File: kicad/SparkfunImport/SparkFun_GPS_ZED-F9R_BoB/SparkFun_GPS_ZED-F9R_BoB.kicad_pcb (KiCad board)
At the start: 2 copper layers, 43.2 x 50.8 mm, 145 parts, among them J1 U.FL, J2 USB_C_2-LAYER_PADS, J3 QWIIC_RIGHT_ANGLE, J4 QWIIC_RIGHT_ANGLE, J5 CONN_111X11_NO_SILK, J6 CONN_09NO_SILK, J7 CONN_06NO_SILK_NO_POP, U1 DUAL-OPTO_HCPL-073L, U2 U-BLOX_ZED_F9R, U3 UHS_INVERTER_SCHMITT_TRIGGERS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, U4 UHS_INVERTER_SCHMITT_TRIGGERS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, U5 V_REG_AP2112K-3.3V

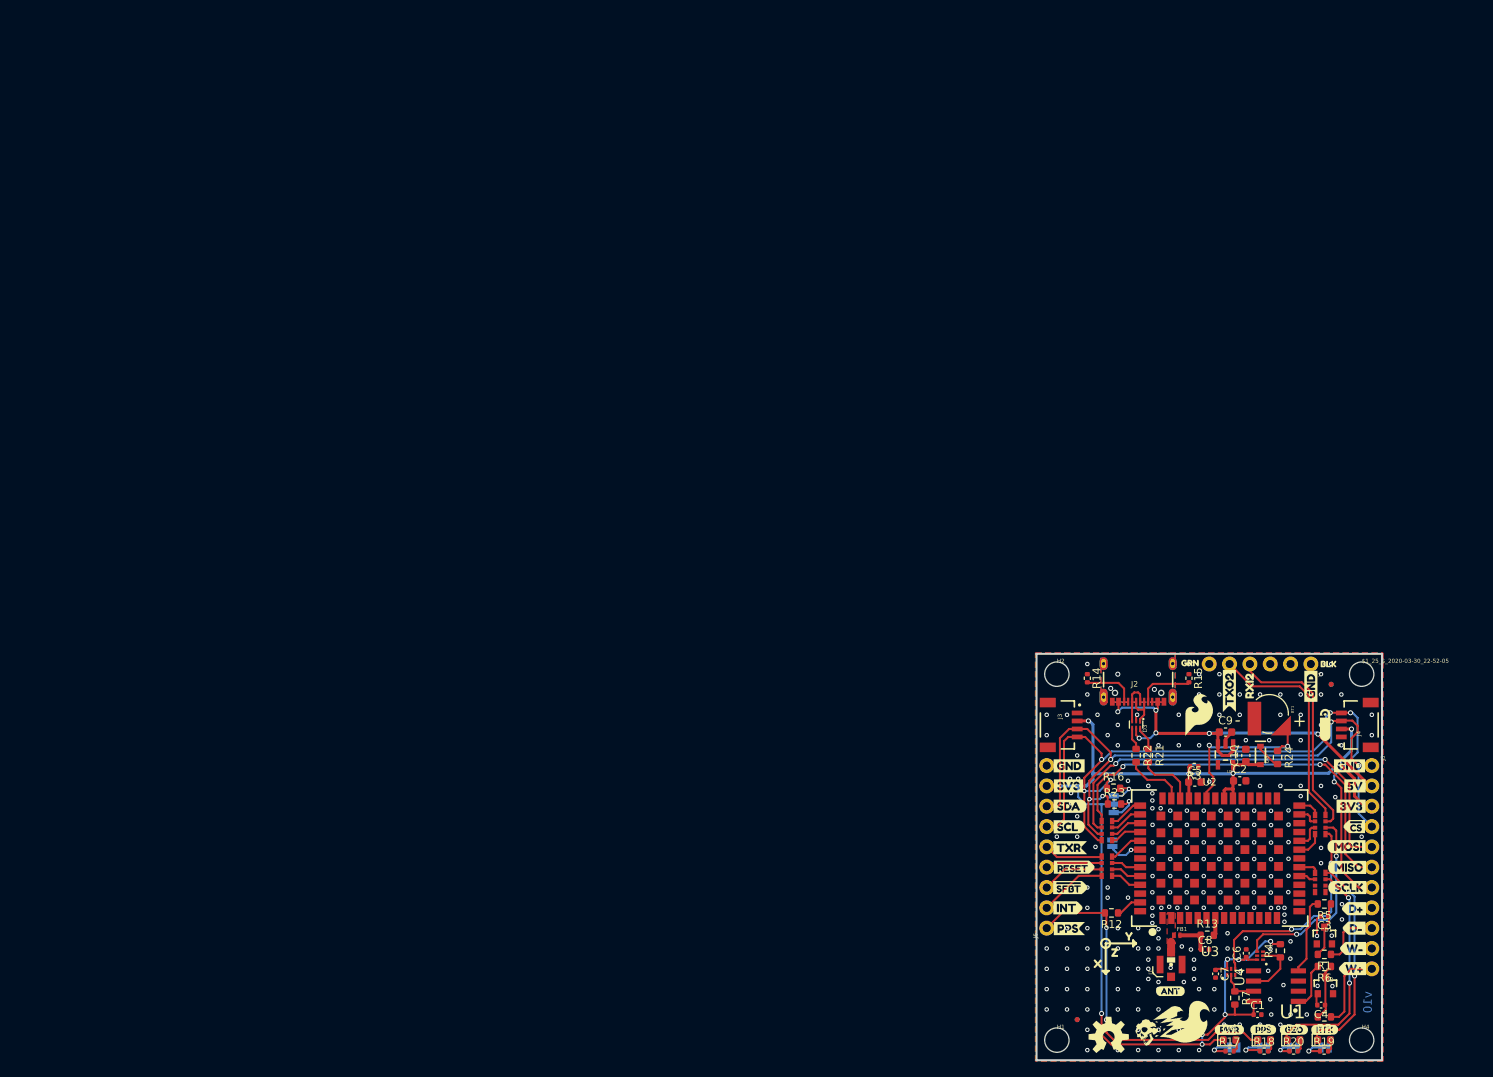
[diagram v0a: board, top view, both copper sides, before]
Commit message: Starting to make gps_breakout
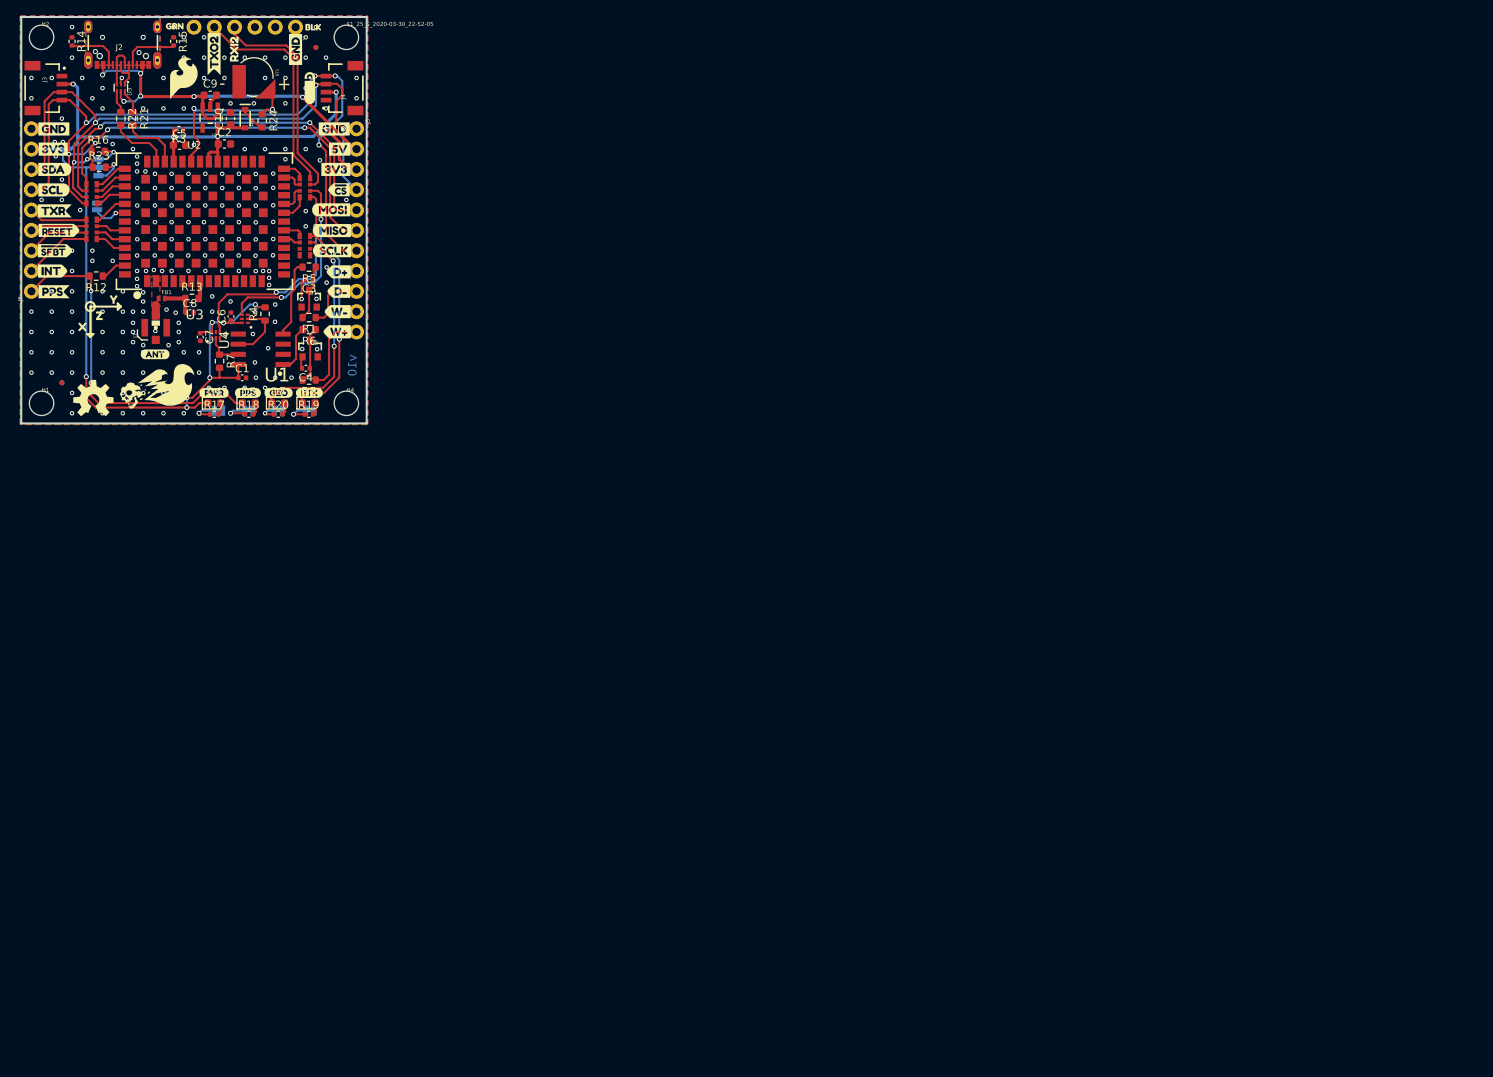
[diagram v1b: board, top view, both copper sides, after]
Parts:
- moved BT1 149.8 mm to (29.1, 7.49)
- moved C1 149.8 mm to (27.6, 45.1)
- moved C10 149.8 mm to (26.2, 12.7)
- moved C2 149.8 mm to (25.4, 15.9)
- moved C3 149.8 mm to (36.0, 32.8)
- moved C4 149.8 mm to (35.6, 43.9)
- moved C5 149.8 mm to (19.8, 16.0)
- moved C6 149.8 mm to (26.2, 37.4)
- moved C8 149.8 mm to (21.1, 37.0)
- moved D1 149.8 mm to (36.0, 35.3)
- moved D2 149.8 mm to (36.1, 41.5)
- moved D3 149.8 mm to (12.4, 8.84)
- moved D4 149.8 mm to (24.1, 48.3)
- moved D5 149.8 mm to (28.4, 48.3)
- moved D6 149.8 mm to (35.9, 48.3)
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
